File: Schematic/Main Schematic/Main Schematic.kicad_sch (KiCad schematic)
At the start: 6 parts, among them J2 Conn_01x24_Socket, J2 Conn_ARM_JTAG_SWD_10, J2 USB_B_Micro, J3 Conn_01x24_Socket, SW2 SW_Push

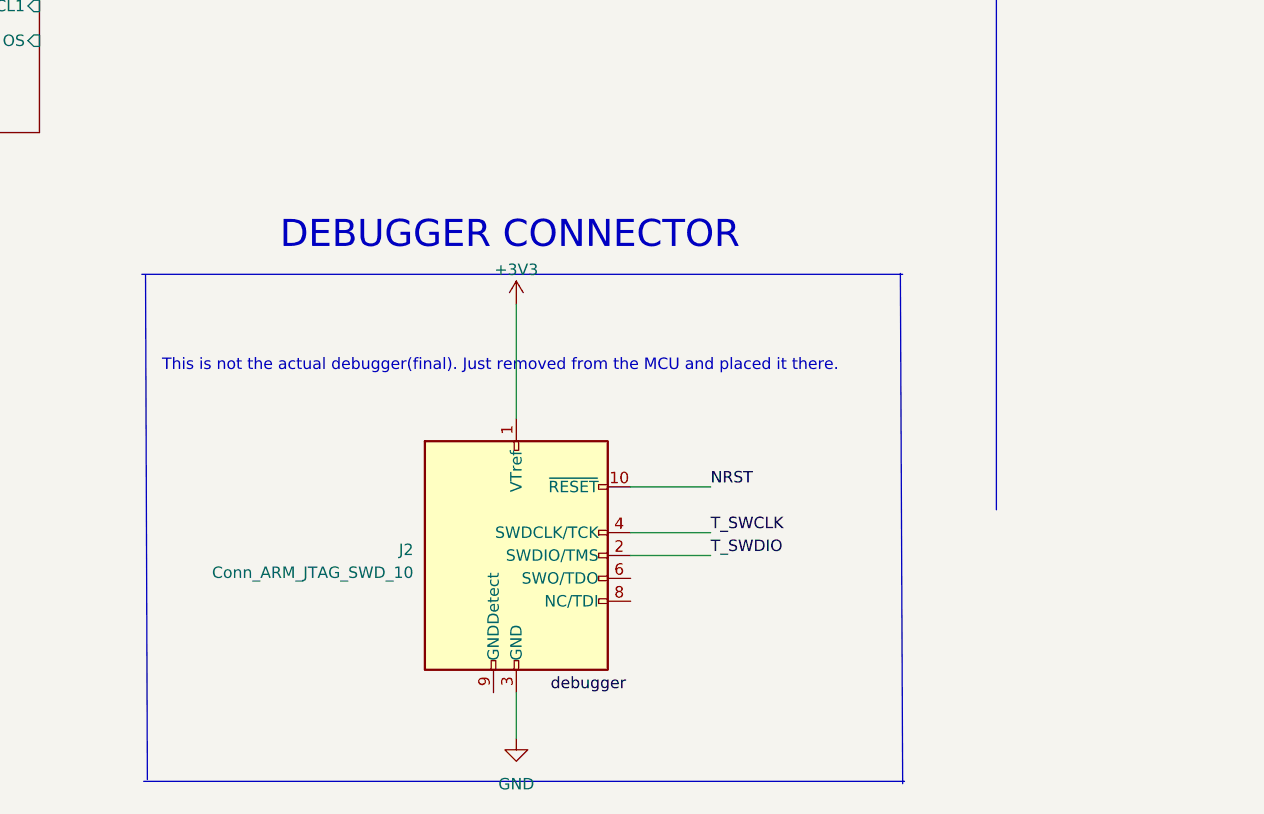
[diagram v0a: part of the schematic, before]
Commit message: 'Updated'
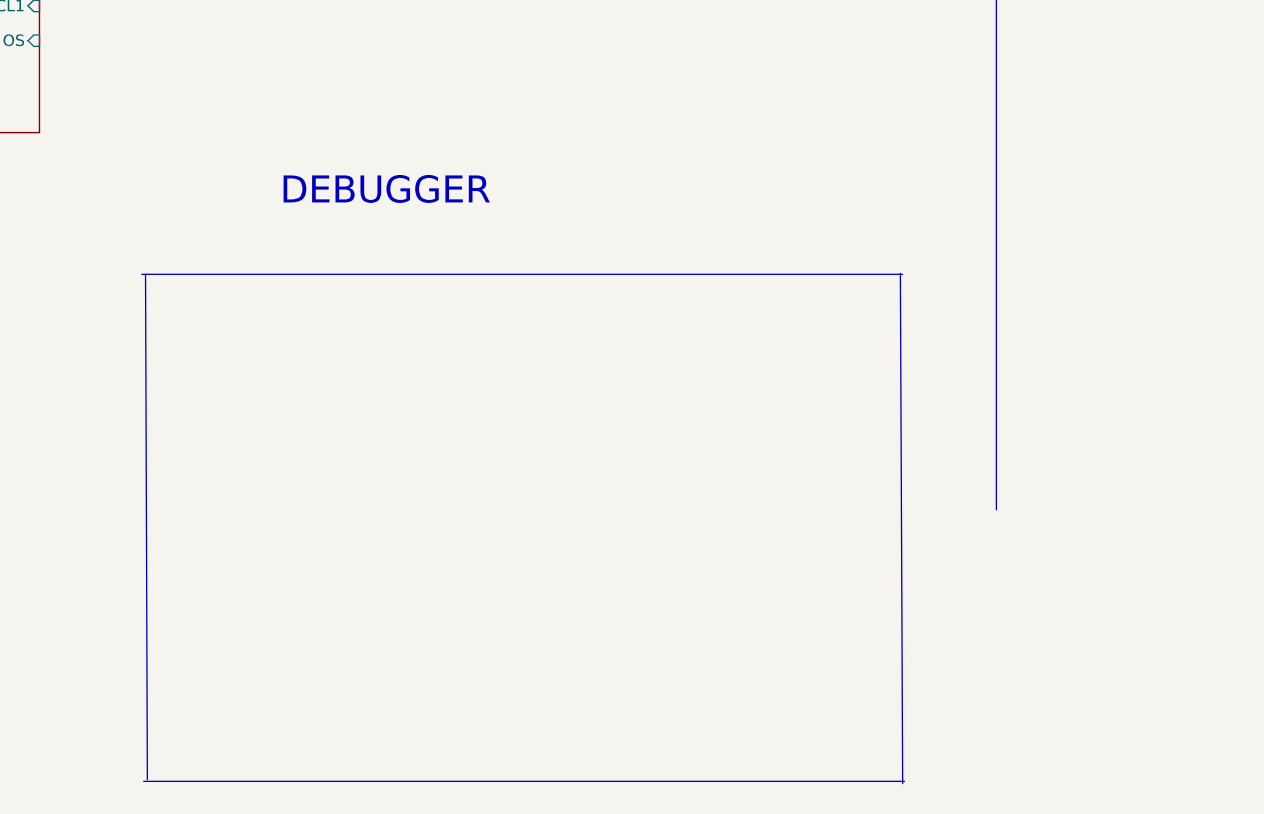
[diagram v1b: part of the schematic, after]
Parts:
- removed J2: Conn_ARM_JTAG_SWD_10, symbol Connector:Conn_ARM_JTAG_SWD_10
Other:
- note added: "DEBUGGER"
- note removed: "DEBUGGER CONNECTOR"
- note removed: "This is not the actual debugger(final). Just removed from the MCU and placed it there."
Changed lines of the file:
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@@
-    (stroke (width 0) (type default))
-  )
-  (wire (pts (xy 130.81 142.24) (xy 130.81 154.94))
     (stroke (width 0) (type default))
   )
@@
     (stroke (width 0) (type default))
   )
-  (wire (pts (xy 143.51 170.18) (xy 152.4 170.18))
-    (stroke (width 0) (type default))
-  )
   (wire (pts (xy 151.2316 45.9232) (xy 151.2316 54.8132))
     (stroke (width 0) (type default))
@@
     (stroke (width 0) (type default))
   )
-  (wire (pts (xy 143.51 167.64) (xy 152.4 167.64))
-    (stroke (width 0) (type default))
-  )
   (wire (pts (xy 250.19 78.74) (xy 255.27 78.74))
     (stroke (width 0) (type default))
@@
     (stroke (width 0) (type default))
   )
-  (wire (pts (xy 143.51 162.56) (xy 152.4 162.56))
-    (stroke (width 0) (type default))
-  )
   (wire (pts (xy 207.01 45.72) (xy 207.01 50.8))
     (stroke (width 0) (type default))
@@
     (stroke (width 0) (type default))
   )
-  (wire (pts (xy 130.81 185.42) (xy 130.81 190.5))
-    (stroke (width 0) (type default))
-  )
   (wire (pts (xy 250.19 63.5) (xy 255.27 63.5))
     (stroke (width 0) (type default))
@@
   (wire (pts (xy 215.9 88.9) (xy 224.79 88.9))
     (stroke (width 0) (type default))
-  )
-  (text "This is not the actual debugger(final). Just removed from the MCU and placed it there."
-    (at 91.44 149.86 0)
-    (effects (font (size 1.27 1.27)) (justify left bottom))
   )
   (text "PIN HEADERS" (at 226.5172 21.9964 0)
     (effects (font (size 3 3)) (justify left bottom))
   )
-  (text "DEBUGGER CONNECTOR\n" (at 104.5464 136.398 0)
+  (text "DEBUGGER\n\n" (at 104.5464 136.398 0)
     (effects (font (size 3 3)) (justify left bottom))
   )
-  (label "debugger" (at 134.62 185.42 0) (fields_autoplaced)
-    (effects (font (size 1.27 1.27)) (justify left bottom))
-  )
-  (label "T_SWDIO" (at 152.4 170.18 0) (fields_autoplaced)
-    (effects (font (size 1.27 1.27)) (justify left bottom))
-  )
-  (label "NRST" (at 152.4 162.56 0) (fields_autoplaced)
-    (effects (font (size 1.27 1.27)) (justify left bottom))
-  )
-  (label "T_SWCLK" (at 152.4 167.64 0) (fields_autoplaced)
-    (effects (font (size 1.27 1.27)) (justify left bottom))
-  )
   (global_label "PC14" (shape input) (at 218.44 35.56 180) (fields_autoplaced)
     (effects (font (size 1.27 1.27)) (justify right))
@@
     (property "Intersheetrefs" "${INTERSHEET_REFS}" (at 20.32 -64.77 0)
       (effects (font (size 1.27 1.27)) hide)
-    )
-  )
-  (symbol (lib_id "power:+3V3") (at 130.81 142.24 0) (unit 1)
-    (in_bom yes) (on_board yes) (dnp no) (fields_autoplaced)
-    (property "Reference" "#PWR017" (at 130.81 146.05 0)
-      (effects (font (size 1.27 1.27)) hide)
-    )
-    (property "Value" "+3V3" (at 130.81 138.43 0)
-      (effects (font (size 1.27 1.27)))
-    )
-    (property "Footprint" "" (at 130.81 142.24 0)
-      (effects (font (size 1.27 1.27)) hide)
-    )
-    (property "Datasheet" "" (at 130.81 142.24 0)
-      (effects (font (size 1.27 1.27)) hide)
-    )
-    (pin "1")
-    (instances
-      (project "Main Schematic"
-        (path "/81c41bad-bb43-41af-b405-18d135a809b1/ae15d31d-f7b4-4051-b9d0-3a01939afe0e"
-          (reference "#PWR017") (unit 1)
-        )
-        (path "/81c41bad-bb43-41af-b405-18d135a809b1"
-          (reference "#PWR017") (unit 1)
-        )
-      )
-      (project "Microcontroller Design"
-        (path "/b8d97438-63f4-433e-afdc-8e43ab7e4842"
-          (reference "#PWR06") (unit 1)
-        )
-      )
-      (project "MCU"
-        (path "/e0666d22-e687-4adb-b95b-6588526d91f1"
-          (reference "#PWR07") (unit 1)
-        )
-      )
     )
   )
@@
         )
       )
-    )
-  )
-  (symbol (lib_id "Connector:Conn_ARM_JTAG_SWD_10") (at 130.81 170.18 0) (unit 1)
-    (in_bom yes) (on_board yes) (dnp no) (fields_autoplaced)
-    (property "Reference" "J2" (at 119.38 169.545 0)
-      (effects (font (size 1.27 1.27)) (justify right))
-    )
-    (property "Value" "Conn_ARM_JTAG_SWD_10" (at 119.38 172.085 0)
-      (effects (font (size 1.27 1.27)) (justify right))
-    )
-    (property "Footprint" "" (at 130.81 170.18 0)
-      (effects (font (size 1.27 1.27)) hide)
-    )
-    (property "Datasheet" "http://infocenter.arm.com/help/topic/com.arm.doc.ddi0314h/DDI0314H_coresight_components_trm.pdf" (at 121.92 201.93 90)
-      (effects (font (size 1.27 1.27)) hide)
-    )
-    (pin "1")
-    (pin "10")
-    (pin "2")
-    (pin "3")
-    (pin "4")
-    (pin "5")
-    (pin "6")
-    (pin "7")
-    (pin "8")
-    (pin "9")
-    (instances
-      (project "Main Schematic"
-        (path "/81c41bad-bb43-41af-b405-18d135a809b1/ae15d31d-f7b4-4051-b9d0-3a01939afe0e"
-          (reference "J2") (unit 1)
-        )
-        (path "/81c41bad-bb43-41af-b405-18d135a809b1"
-          (reference "J4") (unit 1)
-        )
-      )
-      (project "Microcontroller Design"
-        (path "/b8d97438-63f4-433e-afdc-8e43ab7e4842"
-          (reference "J1") (unit 1)
-        )
-      )
-      (project "MCU"
-        (path "/e0666d22-e687-4adb-b95b-6588526d91f1"
-          (reference "J3") (unit 1)
-        )
-      )
-    )
-  )
-  (symbol (lib_id "power:GND") (at 130.81 190.5 0) (unit 1)
-    (in_bom yes) (on_board yes) (dnp no) (fields_autoplaced)
-    (property "Reference" "#PWR018" (at 130.81 196.85 0)
-      (effects (font (size 1.27 1.27)) hide)
-    )
-    (property "Value" "GND" (at 130.81 195.58 0)
-      (effects (font (size 1.27 1.27)))
-    )
-    (property "Footprint" "" (at 130.81 190.5 0)
-      (effects (font (size 1.27 1.27)) hide)
-    )
-    (property "Datasheet" "" (at 130.81 190.5 0)
-      (effects (font (size 1.27 1.27)) hide)
-    )
-    (pin "1")
-    (instances
-      (project "Main Schematic"
-        (path "/81c41bad-bb43-41af-b405-18d135a809b1/ae15d31d-f7b4-4051-b9d0-3a01939afe0e"
-          (reference "#PWR018") (unit 1)
-        )
-        (path "/81c41bad-bb43-41af-b405-18d135a809b1"
-          (reference "#PWR018") (unit 1)
-        )
-      )
-      (project "Microcontroller Design"
-        (path "/b8d97438-63f4-433e-afdc-8e43ab7e4842"
-          (reference "#PWR07") (unit 1)
-        )
-      )
-      (project "MCU"
-        (path "/e0666d22-e687-4adb-b95b-6588526d91f1"
-          (reference "#PWR08") (unit 1)
-        )
-      )
